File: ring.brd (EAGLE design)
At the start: 82.5 x 87.6 mm, 22 parts

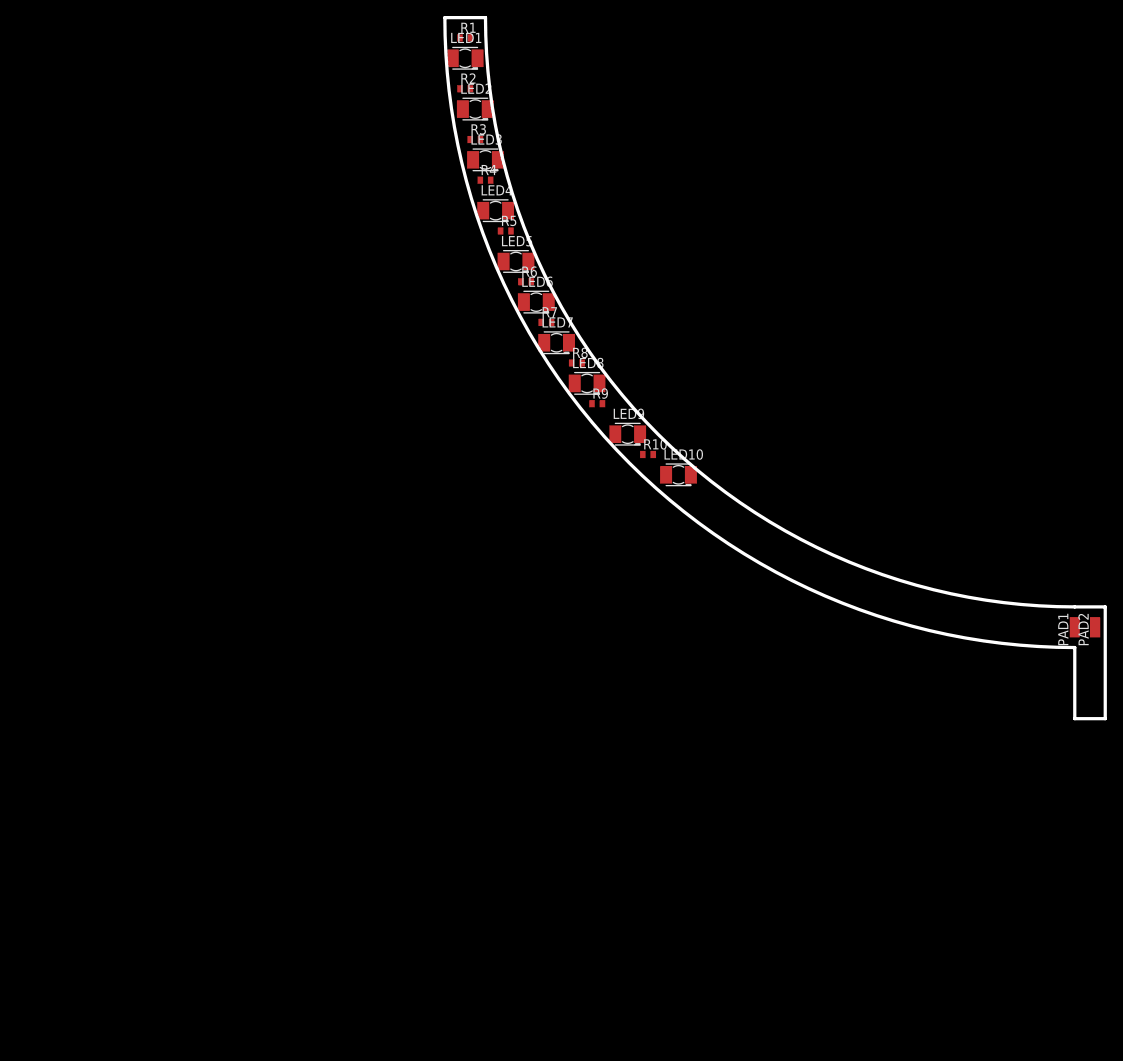
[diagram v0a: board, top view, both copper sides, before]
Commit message: dimensions
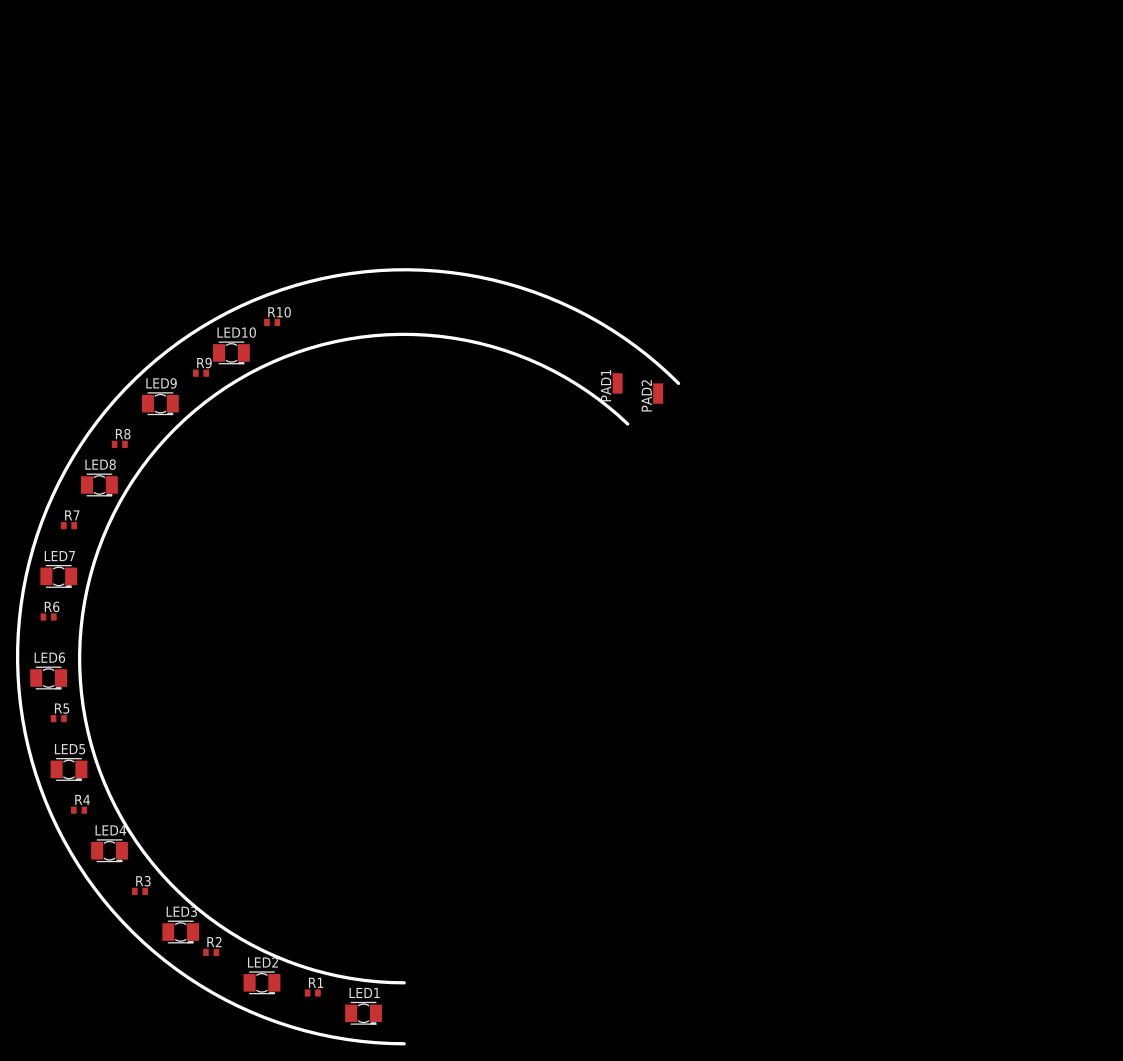
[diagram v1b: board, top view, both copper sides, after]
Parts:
- R1, R10, R2, R3, R4, R5, R6, R7, R8, R9: value (none) -> 330R
- moved R1 120.9 mm to (-11.4, -41.9)
- moved LED1 120.1 mm to (-5.08, -44.5)
- moved R2 112.5 mm to (-24.1, -36.8)
- moved LED2 112.4 mm to (-17.8, -40.6)
- moved LED3 103.8 mm to (-27.9, -34.3)
- moved R3 102.9 mm to (-33.0, -29.2)
- moved R4 93.7 mm to (-40.6, -19.1)
- moved LED4 93.4 mm to (-36.8, -24.1)
- moved LED5 84.6 mm to (-41.9, -14.0)
- moved R5 82.7 mm to (-43.2, -7.62)
- moved LED6 77.0 mm to (-44.5, -2.54)
- moved R6 72.9 mm to (-44.5, 5.08)
- moved LED7 68.7 mm to (-43.2, 10.2)
- moved R7 64.9 mm to (-41.9, 16.5)
- moved PAD1 64.8 mm to (26.7, 34.3)
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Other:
- board size 82.5 x 87.6 mm -> 82.6 x 96.8 mm

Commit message: skog
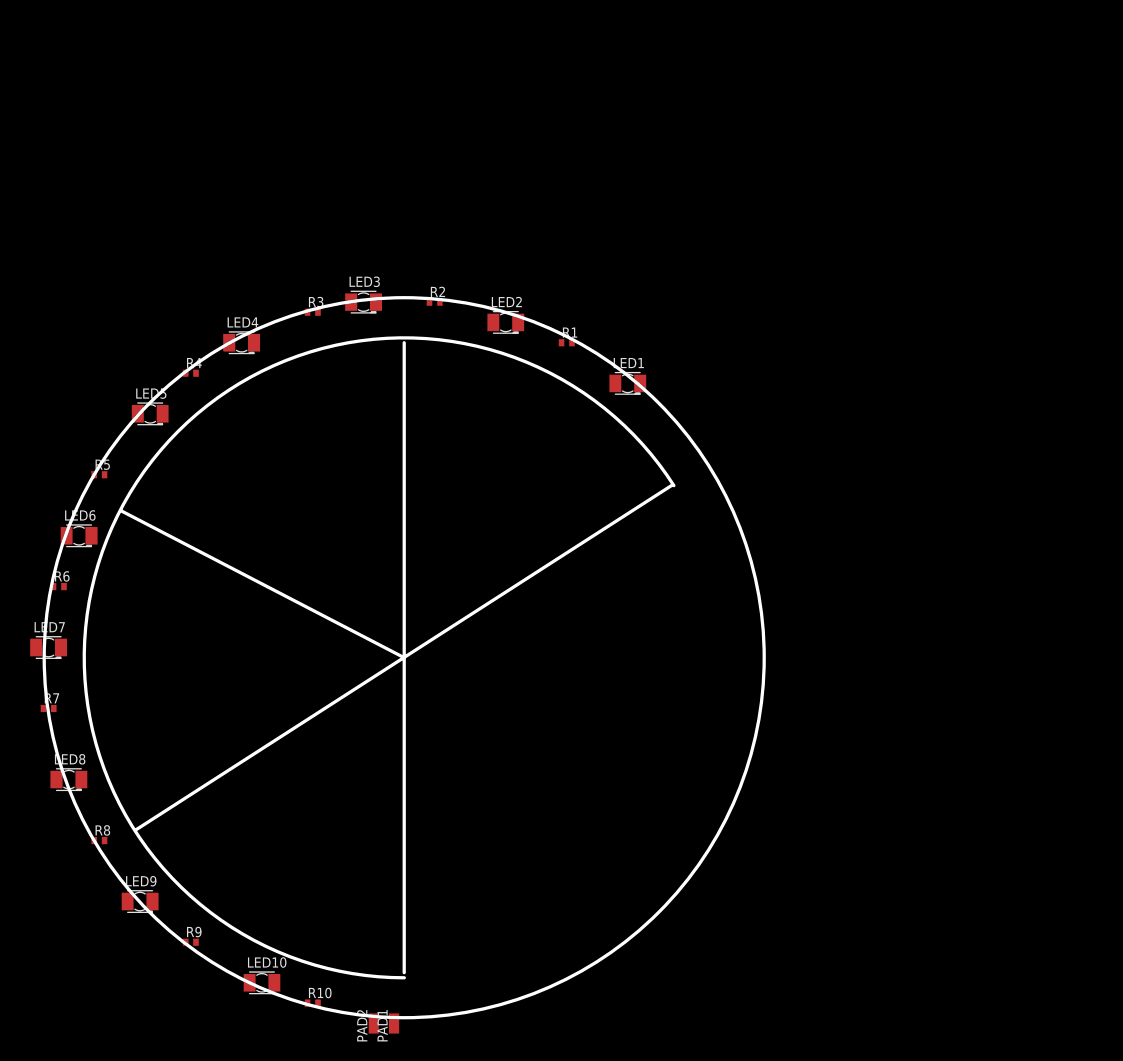
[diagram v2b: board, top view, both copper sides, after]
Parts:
- moved LED2 88.0 mm to (12.7, 41.9)
- moved R1 87.3 mm to (20.3, 39.4)
- moved PAD2 86.4 mm to (-3.81, -45.7)
- moved R2 85.9 mm to (3.81, 44.5)
- moved LED1 85.4 mm to (27.9, 34.3)
- moved R10 85.2 mm to (-11.4, -43.2)
- moved PAD1 84.7 mm to (-1.27, -45.7)
- moved LED3 82.0 mm to (-5.08, 44.5)
- moved LED10 78.8 mm to (-17.8, -40.6)
- moved R3 75.5 mm to (-11.4, 43.2)
- moved R9 71.1 mm to (-26.7, -35.6)
- moved LED4 65.6 mm to (-20.3, 39.4)
- moved LED9 62.3 mm to (-33.0, -30.5)
- moved R4 56.4 mm to (-26.7, 35.6)
- moved R8 49.6 mm to (-38.1, -22.9)
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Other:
- board size 82.6 x 96.8 mm -> 90 x 90 mm
